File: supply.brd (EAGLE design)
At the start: 25.4 x 53.3 mm, 12 parts

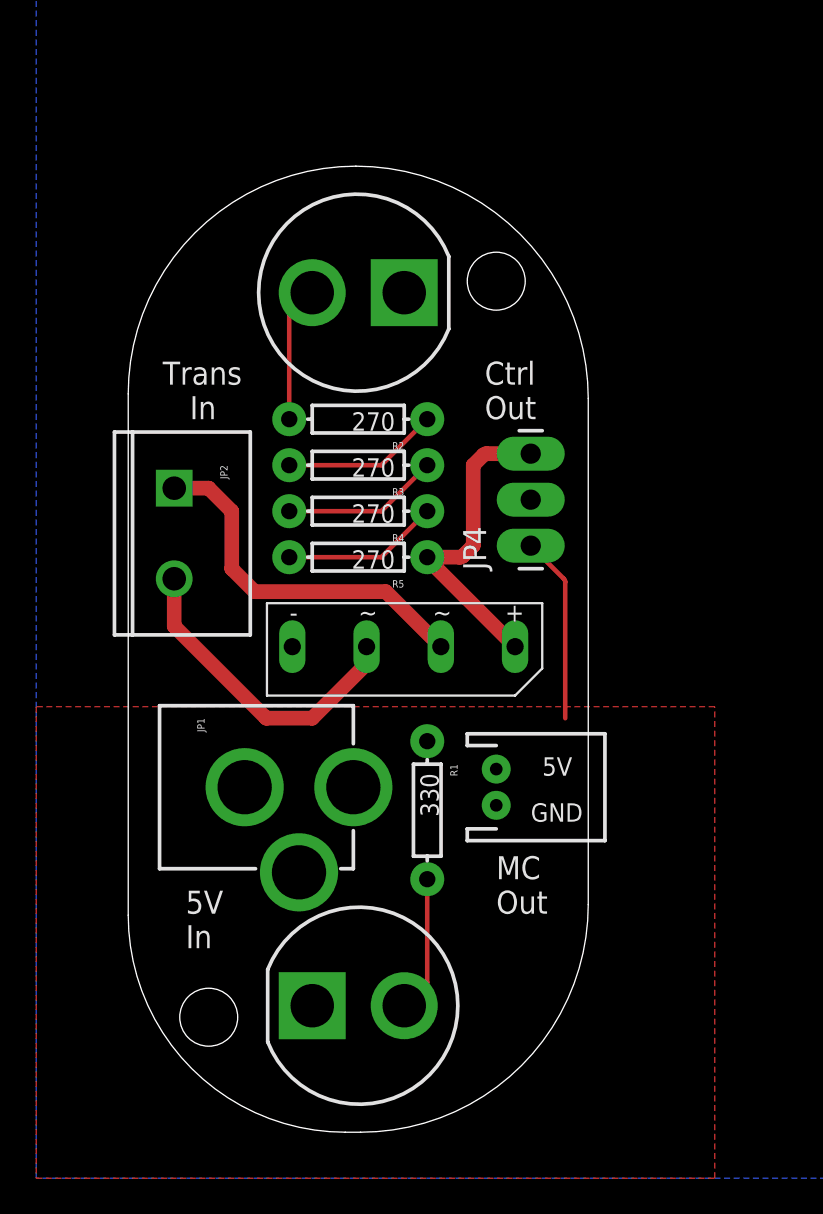
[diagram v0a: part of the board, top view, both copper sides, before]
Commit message: update version and documentation
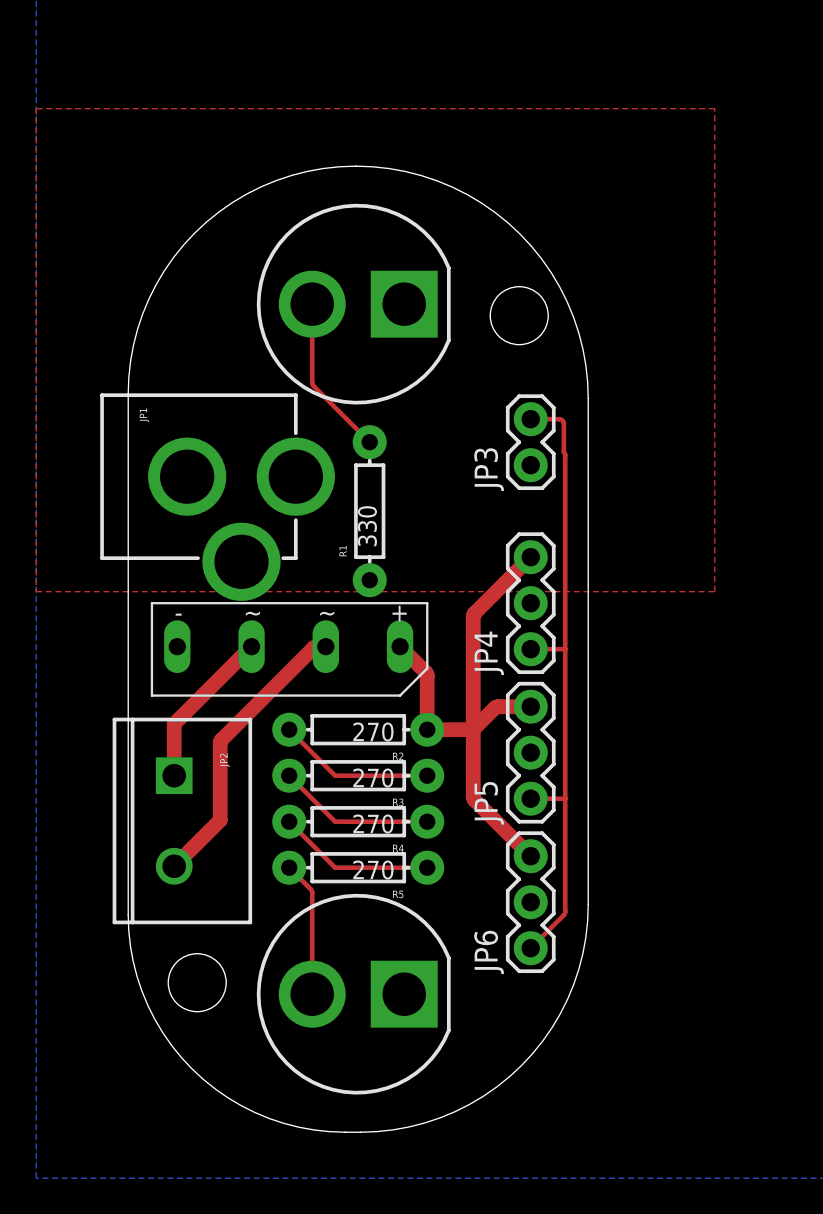
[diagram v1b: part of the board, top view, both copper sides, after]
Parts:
- added JP5, JP6: (no value), SparkFun-Connectors:1X03
- JP3: value M02 -> (none); device custom-parts:JST-2-PTH -> SparkFun-Connectors:1X02
- JP4: device SparkFun-Connectors:1X03_LONGPADS -> SparkFun-Connectors:1X03
- moved D3 38.7 mm to (17.8, 48.3), turned to 180 degrees
- moved D4 38.7 mm to (17.8, 10.2)
- moved JP3 17.9 mm to (27.3, 39.4), turned to 90 degrees
- moved JP1 17.4 mm to (0.64, 38.7)
- moved R4 17.1 mm to (17.8, 19.7)
- moved R5 17.1 mm to (17.8, 17.1)
- moved R2 17.1 mm to (17.8, 24.8)
- moved R3 17.1 mm to (17.8, 22.2)
- moved R1 16.8 mm to (18.4, 36.8), turned to 90 degrees
- moved JP2 15.9 mm to (7.62, 22.2)
- moved U$1 6.35 mm to (21.6, 31.8)
- moved JP4 5.71 mm to (27.3, 29.2)
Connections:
- net 5V: now also JP3.2, JP5.1, JP6.1; no longer JP3.1
- net GND: now also JP3.1, JP5.2, JP6.2; no longer JP3.2
- net I1: now also JP2.2; no longer JP2.1
- net I2: now also JP2.1; no longer JP2.2
- net N$1: now also R2.P$2, R3.P$1; no longer R2.P$1, R3.P$2
- net N$2: now also D4.A, R5.P$2; no longer R3.P$1, R4.P$2
- net N$3: now also R3.P$2, R4.P$1; no longer D4.A, R2.P$2
- net N$5: now also R4.P$2, R5.P$1; no longer R4.P$1, R5.P$2
- net V+: now also JP5.3, JP6.3, R2.P$1; no longer R5.P$1
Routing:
- net 5V: track 10.3 -> 35.5 mm
- net V+: track 17.6 -> 30.5 mm
- net I2: track 17.5 -> 8.89 mm
- net I1: track 20.2 -> 15.9 mm
- net N$4: track 7.51 -> 8.92 mm
- net N$2: track 8.67 -> 7.50 mm
- net N$3: track 7.51 -> 8.67 mm
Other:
- board text removed: "5V"
- board text removed: "5V In"
- board text removed: "Ctrl Out"
- board text removed: "GND"
- board text removed: "MC Out"
- board text removed: "Trans In"
- board text removed: "V+"
